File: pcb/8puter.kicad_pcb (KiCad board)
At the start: 2 copper layers, 180 x 120 mm, 88 parts, among them J1 PWR-DC, J2 DB9_Female, J3 USB_A, J4 FPGA_Prog, SW1 RESET_SW, U11 74AC14, U12 W65C22NxPL, U13 MX25V8035F, U14 FT240XQ, U15 LCMXO2-256ZE-3SG32I, U2 74AHC74, U3 DS1135Z-6+, U6 MAX811MEUS-T, U7 STM8S003K3T, U8 74AHC00

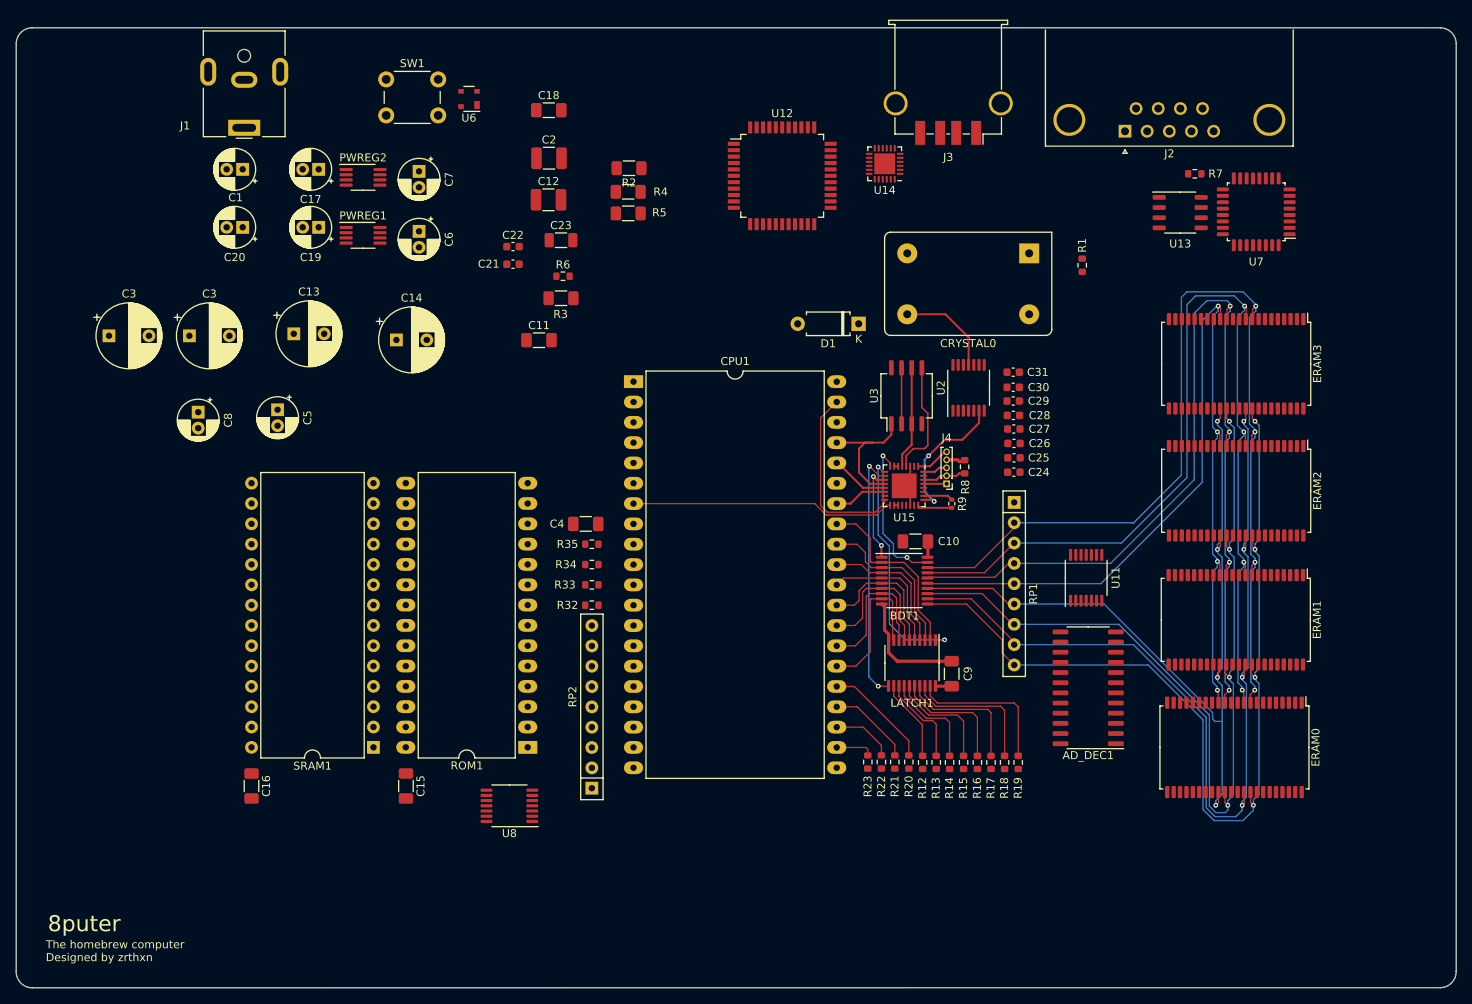
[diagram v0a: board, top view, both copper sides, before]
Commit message: Serial interface
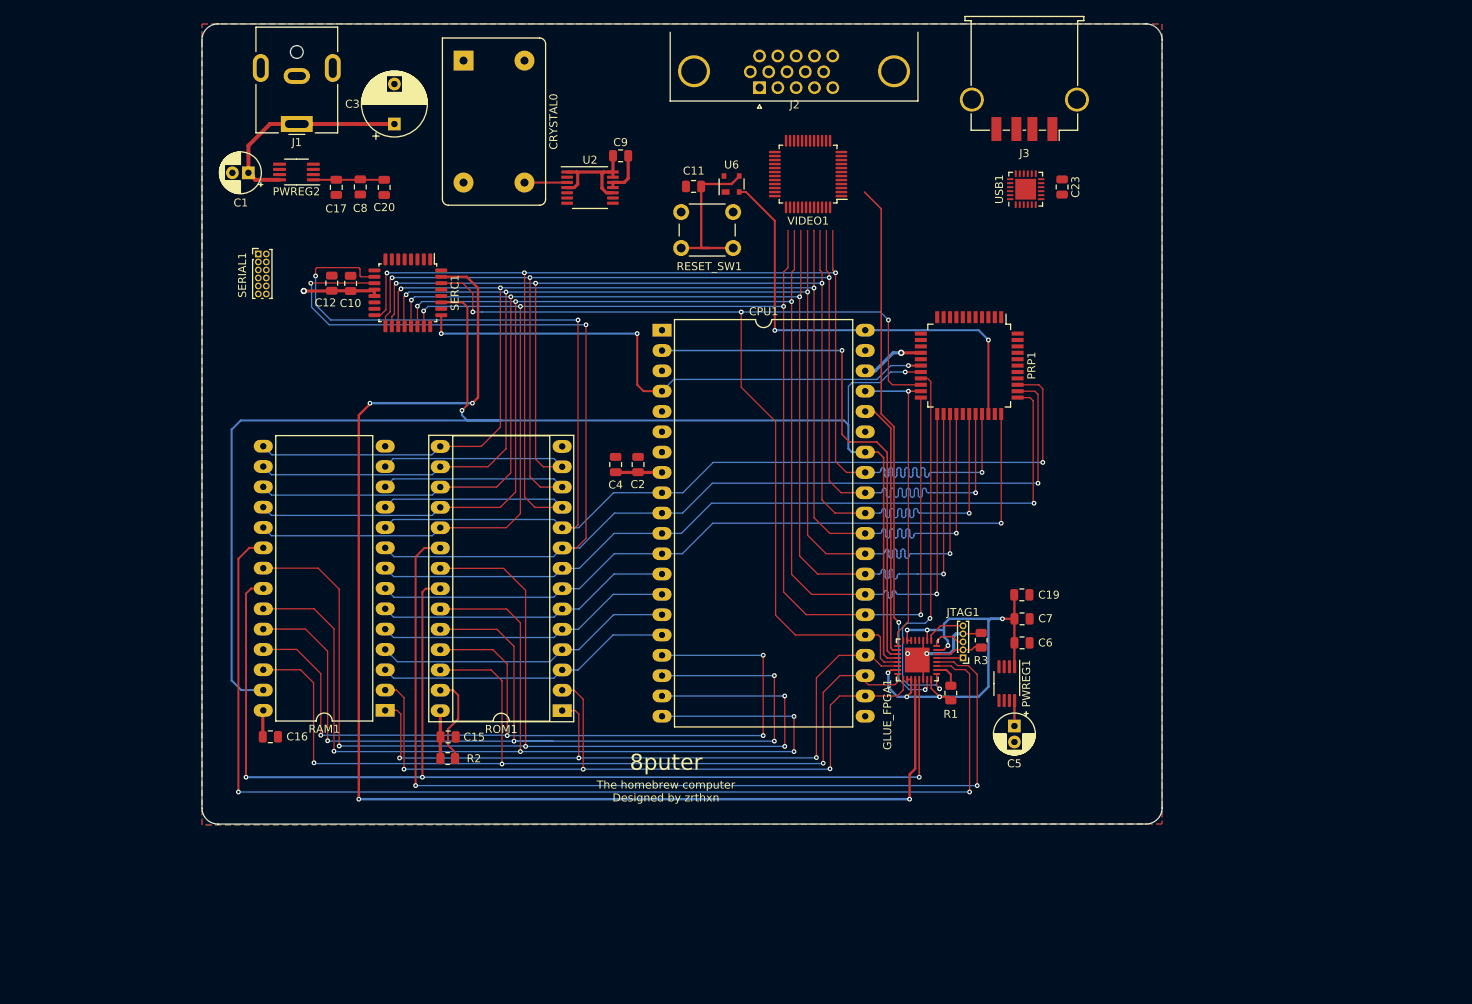
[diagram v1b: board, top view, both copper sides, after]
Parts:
- removed AD_DEC1: 74HCT154, Package_SO:SO-24_5.3x15mm_P1.27mm
- removed BDT1: 74AC245, Package_SO:TSSOP-20_4.4x6.5mm_P0.65mm
- removed C13, C14: 1uF, Capacitor_THT:CP_Radial_D8.0mm_P3.80mm
- removed C18: 100nF, Capacitor_SMD:C_1206_3216Metric_Pad1.33x1.80mm_HandSolder
- removed C21, C24, C25, C26, C28: 100nF, Capacitor_SMD:C_0603_1608Metric
- removed C22, C27, C29, C30, C31: 10nF, Capacitor_SMD:C_0603_1608Metric
- removed the C3 at (77.1, 74.2)
- removed the C3 at (87.1, 74.2)
- removed D1: 1N5817, Diode_THT:D_A-405_P7.62mm_Horizontal
- removed ERAM0, ERAM1, ERAM2, ERAM3: IS62WV10248, Package_SO:TSOP-II-44_10.16x18.41mm_P0.8mm
- removed J4: FPGA_Prog, Connector_PinHeader_1.00mm:PinHeader_1x05_P1.00mm_Vertical
- removed LATCH1: 74AC573, Package_SO:TSSOP-20_4.4x6.5mm_P0.65mm
- removed R12, R13, R14, R15, R16, R17, R18, R19, R20, R21, R22, R23, R32, R33, R34, R35, R6, R7: 1K, Resistor_SMD:R_0603_1608Metric
- removed R4, R5: 10K, Resistor_SMD:R_1206_3216Metric_Pad1.30x1.75mm_HandSolder
- removed R8: 4.7K, Resistor_SMD:R_0603_1608Metric
- removed R9: 1K, Resistor_SMD:R_0402_1005Metric
- removed RP1, RP2: 1K, Resistor_THT:R_Array_SIP9
- removed SRAM1: AS6C62256-55PCN, Package_DIP:DIP-28_W15.24mm
- removed SW1: RESET_SW, Button_Switch_THT:SW_PUSH_6mm_H13mm
- removed U11: 74AC14, Package_SO:TSSOP-14_4.4x5mm_P0.65mm
- removed U12: W65C22NxPL, Package_QFP:PQFP-44_10x10mm_P0.8mm
- removed U13: MX25V8035F, Package_SO:SOP-8_3.9x4.9mm_P1.27mm
- removed U14: FT240XQ, Package_DFN_QFN:QFN-24-1EP_4x4mm_P0.5mm_EP2.6x2.6mm
- removed U15: LCMXO2-256ZE-3SG32I, Package_DFN_QFN:QFN-32-1EP_5x5mm_P0.5mm_EP3.1x3.1mm
- removed U3: DS1135Z-6+, Package_SO:SO-8_5.3x6.2mm_P1.27mm
- removed U7: STM8S003K3T, Package_QFP:LQFP-32_7x7mm_P0.8mm
- removed U8: 74AHC00, Package_SO:TSSOP-14_4.4x5mm_P0.65mm
- added C3: 10uF 16V, Capacitor_THT:CP_Radial_D8.0mm_P5.00mm, F.Cu at (112.7, 47.8)
- added GLUE_FPGA1: LCMXO2-256-QFN32, Package_DFN_QFN:QFN-32-1EP_5x5mm_P0.5mm_EP3.1x3.1mm, F.Cu at (178.1, 114.8)
- added JTAG1: PIN_HDR, Connector_PinHeader_1.00mm:PinHeader_1x05_P1.00mm_Vertical, F.Cu at (183.8, 114.5)
- added PRP1: W65C22SxQ, Package_QFP:PQFP-44_10x10mm_P0.8mm, F.Cu at (184.6, 78.0)
- added RAM1: AS6C62256-55PCN, Package_DIP:DIP-28_W15.24mm_LongPads, F.Cu at (111.6, 121.1)
- added RESET_SW1: PUSHBTN, Button_Switch_THT:SW_PUSH_6mm_H13mm, F.Cu at (148.6, 58.8)
- added SERC1: W65C51NxQ, Package_QFP:LQFP-32_7x7mm_P0.8mm, F.Cu at (114.4, 68.9)
- added SERIAL1: Conn_2Rows-11Pins, Connector_PinHeader_1.00mm:PinHeader_2x06_P1.00mm_Vertical, F.Cu at (95.7, 64.0)
- added USB1: FT240XQ, Package_DFN_QFN:QFN-24-1EP_4x4mm_P0.5mm_EP2.6x2.6mm, F.Cu at (191.6, 55.9)
- added VIDEO1: STM32F301C6Tx, Package_QFP:LQFP-48_7x7mm_P0.5mm, F.Cu at (164.4, 54.0)
- C10, C11, C15, C16, C4, C9: footprint Capacitor_SMD:C_1206_3216Metric_Pad1.33x1.80mm_HandSolder -> Capacitor_SMD:C_0805_2012Metric
- C12: value 1uF -> 100nF; footprint Capacitor_SMD:C_1210_3225Metric_Pad1.33x2.70mm_HandSolder -> Capacitor_SMD:C_0805_2012Metric
- C17, C19, C20, C6, C7, C8: footprint Capacitor_THT:CP_Radial_D5.0mm_P2.00mm -> Capacitor_SMD:C_0805_2012Metric
- C2: footprint Capacitor_SMD:C_1210_3225Metric_Pad1.33x2.70mm_HandSolder -> Capacitor_SMD:C_0805_2012Metric
- C23: footprint Capacitor_SMD:C_1206_3216Metric -> Capacitor_SMD:C_0805_2012Metric
- CPU1: value W65C816SxP -> W65C02SxP
- J2: value DB9_Female -> DB15_Female; footprint Connector_Dsub:DSUB-9_Female_Horizontal_P2.77x2.84mm_EdgePinOffset9.90mm_Housed_MountingHolesOffset11.32mm -> Connector_Dsub:DSUB-15-HD_Female_Horizontal_P2.29x1.98mm_EdgePinOffset3.03mm_Housed_MountingHolesOffset4.94mm
- R1: footprint Resistor_SMD:R_0603_1608Metric -> Resistor_SMD:R_0805_2012Metric
- R2: footprint Resistor_SMD:R_1206_3216Metric_Pad1.30x1.75mm_HandSolder -> Resistor_SMD:R_0805_2012Metric
- R3: value 10K -> 4.7K; footprint Resistor_SMD:R_1206_3216Metric_Pad1.30x1.75mm_HandSolder -> Resistor_SMD:R_0805_2012Metric
- ROM1: footprint Package_DIP:DIP-28_W15.24mm_LongPads -> Package_DIP:DIP-28_W15.24mm_Socket_LongPads
- moved C5 100.2 mm to (190.2, 123.0)
- moved C19 99.2 mm to (191.2, 106.6), turned to 0 degrees
- moved PWREG1 98.1 mm to (189.3, 117.7), turned to -90 degrees
- moved C7 93.9 mm to (191.2, 109.6), turned to 0 degrees
- moved C6 91.3 mm to (191.2, 112.6), turned to 0 degrees
- moved C10 77.6 mm to (107.3, 67.7), turned to -90 degrees
- moved R2 77.2 mm to (119.4, 127.1), turned to 0 degrees
- moved C9 76.8 mm to (141.0, 51.7), turned to 0 degrees
- moved CRYSTAL0 74.7 mm to (121.4, 39.8), turned to -90 degrees
- moved R3 67.7 mm to (186.1, 112.3), turned to 90 degrees
- moved C23 63.0 mm to (196.2, 55.6), turned to -90 degrees
- moved R1 55.9 mm to (182.3, 118.9)
- moved U2 53.5 mm to (137.2, 55.7), turned to 0 degrees
- moved J2 46.0 mm to (158.4, 43.2)
- moved C2 39.9 mm to (143.2, 90.3), turned to 90 degrees
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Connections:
- net RESET renamed ~{RESET}
- C10 pad 1: +5V -> GND
- C10 pad 2: GND -> +5V
- C12 pad 1: +5V -> GND
- C12 pad 2: GND -> +5V
- C19 pad 1: Net-(C19-Pad1) -> +3V3
- C5 pad 1: /Power/PWR -> +5V
- C6 pad 1: Net-(C19-Pad1) -> +3V3
- C7 pad 1: Net-(C19-Pad1) -> +3V3
- CPU1 pad 26: /DBA7 -> DATA7
- CPU1 pad 27: /DBA6 -> DATA6
- CPU1 pad 28: /DBA5 -> DATA5
- CPU1 pad 29: /DBA4 -> DATA4
- CPU1 pad 3: Net-(CPU1-Pad3) -> unconnected-(CPU1-Pad3)
- CPU1 pad 30: /DBA3 -> DATA3
- CPU1 pad 31: /DBA2 -> DATA2
- CPU1 pad 32: /DBA1 -> DATA1
- CPU1 pad 33: /DBA0 -> DATA0
- CPU1 pad 35: EMU -> unconnected-(CPU1-Pad35)
- CPU1 pad 38: unconnected-(CPU1-Pad38) -> +5V
- CPU1 pad 39: VDA -> unconnected-(CPU1-Pad39)
- CPU1 pad 7: VPA -> unconnected-(CPU1-Pad7)
- J3 pad 2: unconnected-(J3-Pad2) -> Net-(J3-Pad2)
- J3 pad 3: unconnected-(J3-Pad3) -> Net-(J3-Pad3)
- J3 pad 4: unconnected-(J3-Pad4) -> GND
- J3 pad 5: unconnected-(J3-Pad5) -> GND
- PWREG1 pad 1: Net-(C19-Pad1) -> +3V3
- PWREG1 pad 4: unconnected-(PWREG1-Pad4) -> GND
- PWREG1 pad 8: /Power/PWR -> +5V
- R1 pad 1: +5V -> Net-(R1-Pad1)
- R1 pad 2: RDY -> +3V3
- R3 pad 1: +5V -> /TCK
- R3 pad 2: Net-(R3-Pad2) -> GND
- ROM1 pad 20: /Memory Unit/~{ROM_CS} -> ~{RAM_CS}
- ROM1 pad 22: ~{READ} -> CPU_W~{R}
- U2 pad 11: /Clock/CRYSTAL -> GND
- U2 pad 12: ~{CLOCK} -> GND
- U2 pad 14: (no net) -> +5V
- U2 pad 2: Net-(R3-Pad2) -> ~{CLOCK}
- U2 pad 3: /Bus Control/CLK= -> /Clock/CRYSTAL
- U2 pad 5: /Bus Control/RDY_R -> CLOCK
- U2 pad 6: /Bus Control/~{RDY_R} -> ~{CLOCK}
- U2 pad 7: (no net) -> GND
- U2 pad 8: ~{CLOCK} -> unconnected-(U2-Pad8)
- U2 pad 9: CLOCK -> unconnected-(U2-Pad9)
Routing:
- net CPU_R~{W}: track 6.61 -> 185.1 mm, vias 0 -> 2
- net ADDR1: track 0.00 -> 176.1 mm, vias 0 -> 3
- net ADDR0: track 0.00 -> 173.2 mm, vias 0 -> 3
- net ~{SERIAL_CS}: track 0.00 -> 166.8 mm, vias 0 -> 4
- net CPU_W~{R}: track 0.00 -> 147.3 mm, vias 0 -> 3
- net ~{ROM_CS}: track 0.00 -> 143.5 mm, vias 0 -> 2
- net ADDR10: track 0.00 -> 139.0 mm, vias 0 -> 4
- net ADDR11: track 0.00 -> 130.4 mm, vias 0 -> 4
- net ADDR9: track 0.00 -> 125.3 mm, vias 0 -> 4
- net ~{RAM_CS}: track 0.00 -> 121.9 mm, vias 0 -> 2
- net ADDR15: track 13.6 -> 130.2 mm, vias 0 -> 3
- net ADDR13: track 7.78 -> 120.5 mm, vias 0 -> 3
- net ADDR8: track 0.00 -> 112.2 mm, vias 0 -> 4
- net ADDR2: track 0.00 -> 100.3 mm, vias 0 -> 1
- net ADDR3: track 0.00 -> 94.9 mm, vias 0 -> 1
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- added copper zone on B.Cu, net +5V
- added copper zone on F.Cu, net GND
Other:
- board size 180 x 120 mm -> 120 x 100 mm
